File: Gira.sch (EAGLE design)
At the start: 25 parts, among them IC1 MEGA8-PTQFP, Q2 2N7002

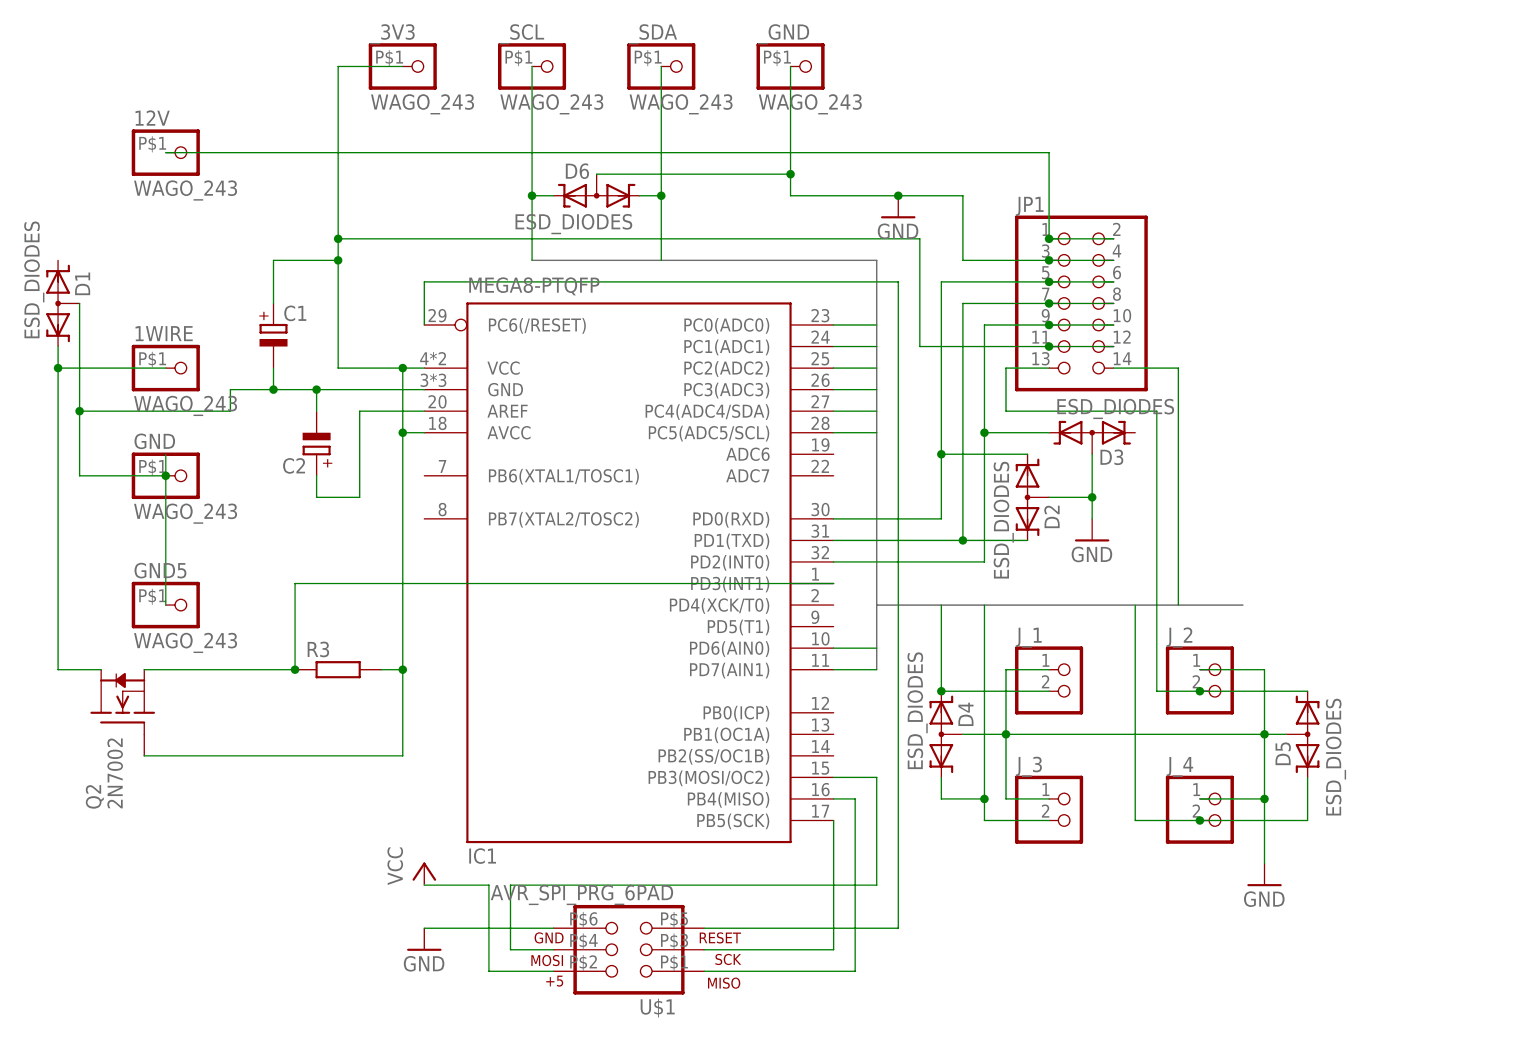
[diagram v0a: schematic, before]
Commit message: V2.2
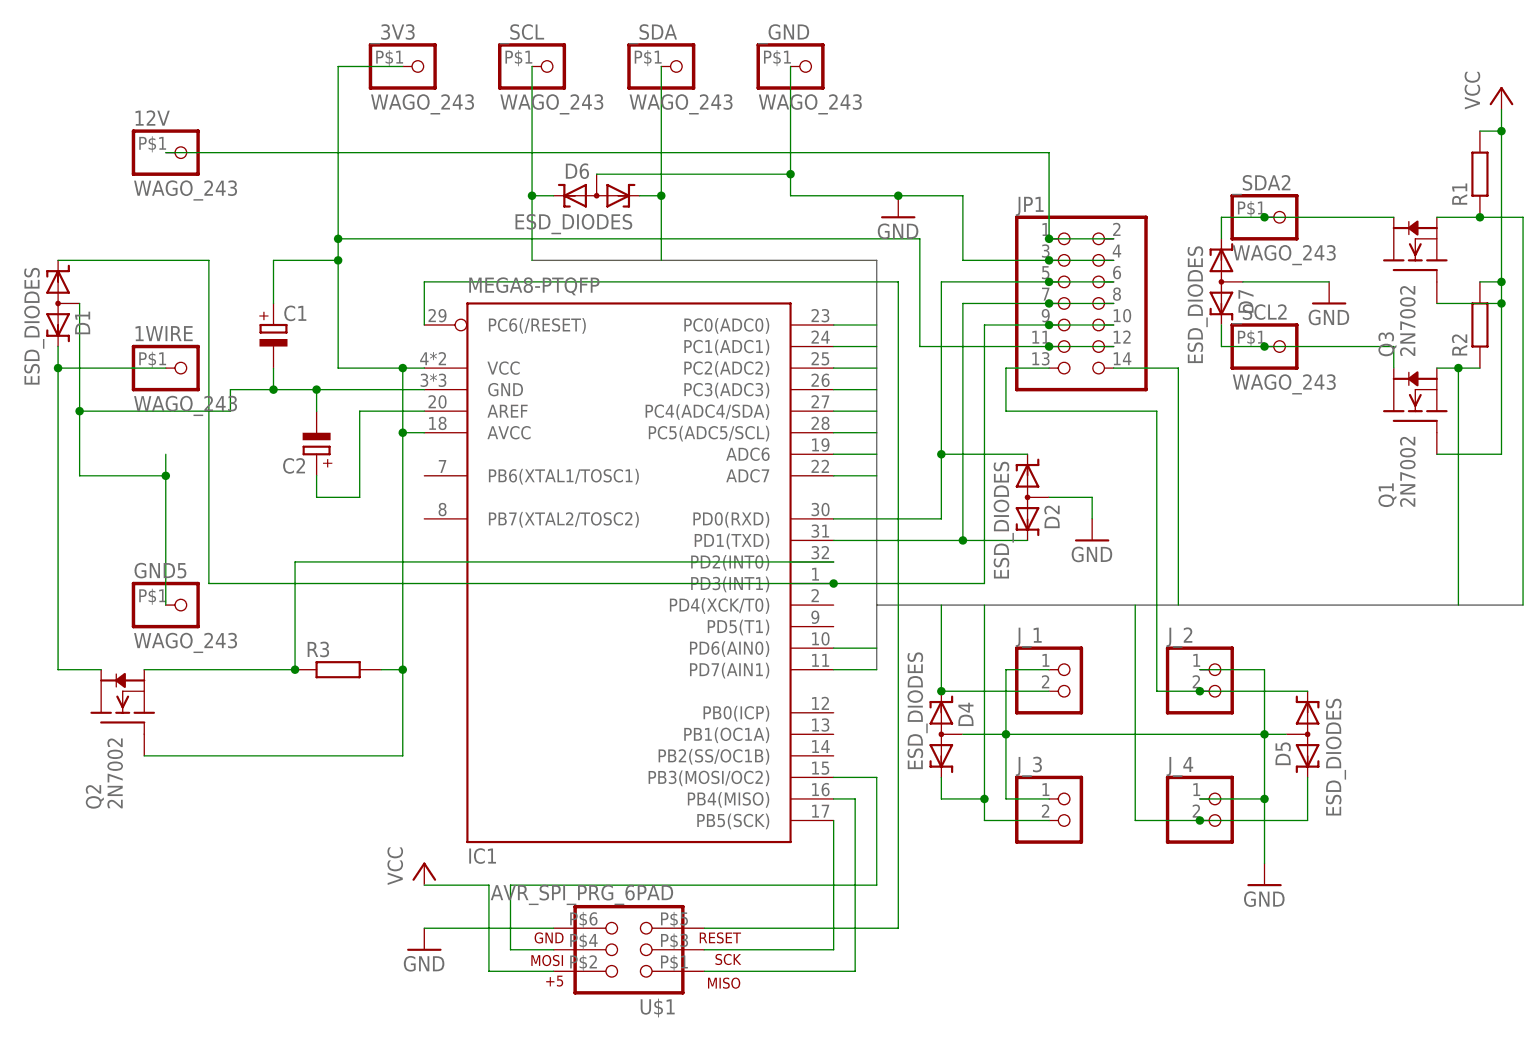
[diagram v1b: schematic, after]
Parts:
- removed D3: ESD_DIODES, common:ESD_DIODES
- removed GND: WAGO_243, common:WAGO_243
- added D7: ESD_DIODES, common:ESD_DIODES
- added Q1, Q3: 2N7002, common:2N7002
- added R1, R2: (no value), common:R-EU_R0603
- added _SCL2, _SDA2: WAGO_243, common:WAGO_243
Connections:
- new net N$4: D7.K1, Q3.D, _SDA2.1
- new net N$5: D7.K2, Q1.D, _SCL2.1
- new net SCL2: IC1.PC5(ADC5/SCL), Q1.S, R2.1
- new net SDA2: IC1.PC4(ADC4/SDA), Q3.S, R1.1
- new net VCC: Q1.G, Q3.G, R1.2, R2.2
- net GND: now also D7.AA; no longer D3.AA, GND.1
- net N$16: now also D1.K1, IC1.PD3(INT1); no longer D3.K1, IC1.PD2(INT0)
- net N$2: now also IC1.PD2(INT0); no longer IC1.PD3(INT1)
- net N$3: now also D1.K2; no longer D1.K1
- net SCL: now also IC1.ADC7; no longer IC1.PC5(ADC5/SCL)
- net SDA: now also IC1.ADC6; no longer IC1.PC4(ADC4/SDA)
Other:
- moved on the sheet: D1
